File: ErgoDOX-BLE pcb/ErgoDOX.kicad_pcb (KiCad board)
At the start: 2 copper layers, 182.8 x 158.9 mm, 110 parts, among them J1 Conn_01x04, J2 Conn_01x02_Female, J3 Conn_01x02_Female, J4 Conn_01x02, J5 Conn_01x02, P1 USB_C_Plug_USB2.0, Q1 Q_NPN_BCE, SW0:10 SW0:3, SW0:11 SW0:2, SW0:12 SW0:1, SW0:7 SW0:6, SW0:8 SW0:5, SW0:9 SW0:4, SW1:10 SW1:3, SW1:11 SW1:2, SW1:12 SW1:1, SW1:13 SW1:0, SW1:9 SW1:4, SW2:10 SW2:3, SW2:11 SW2:2, SW2:12 SW2:1, SW2:13 SW2:0, SW2:7 SW2:6, SW2:8 SW2:5, SW2:9 SW2:4, SW3:10 SW3:3, SW3:11 SW3:2, SW3:12 SW3:1, SW3:13 SW3:0, SW3:8 SW3:5, SW3:9 SW3:4, SW4:10 SW4:3, SW4:11 SW4:2, SW4:12 SW4:1, SW4:13 SW4:0, SW4:7 SW4:6, SW4:8 SW4:5, SW4:9 SW4:4, SW5:10 SW5:3, SW5:11 SW5:2, SW5:12 SW5:1, SW5:13 SW5:0, SW5:7 SW5:6, SW5:8 SW5:5, SW5:9 SW5:4, U1 MCP23018, U3 C0720B001F

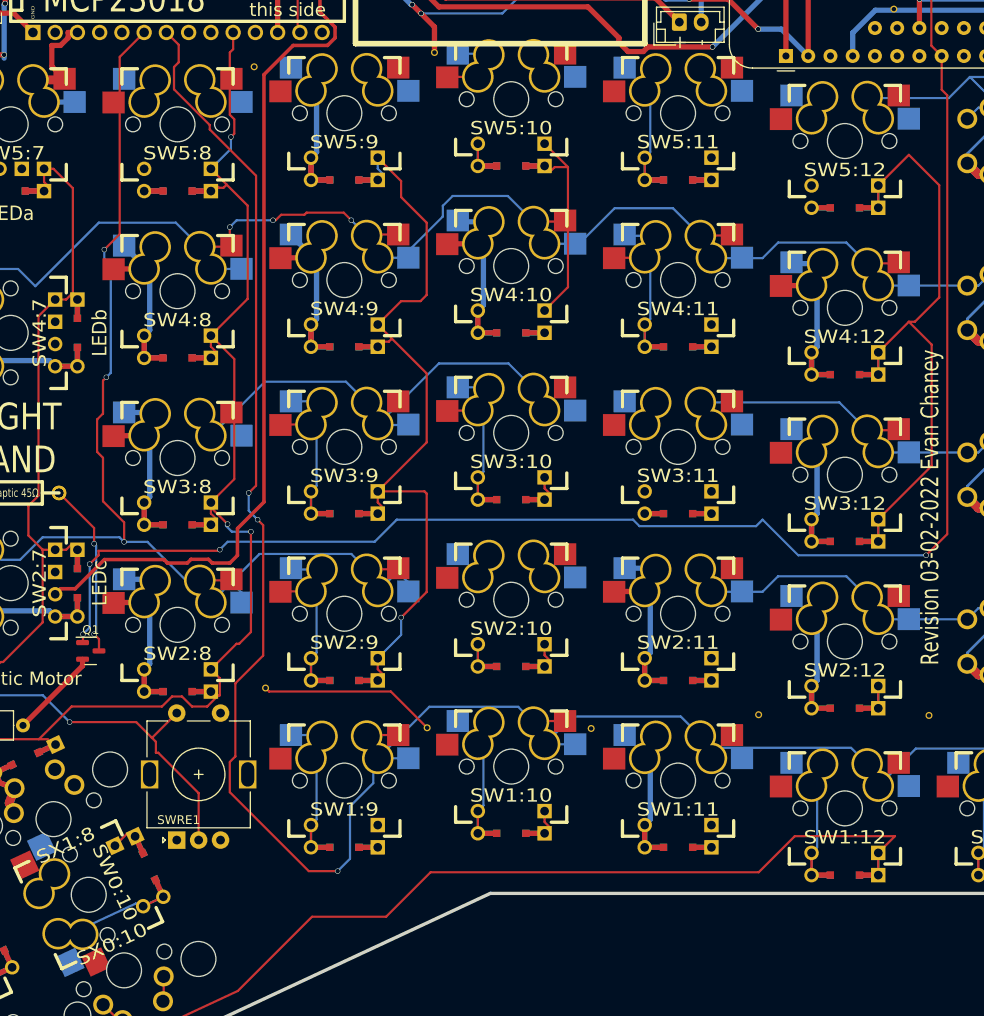
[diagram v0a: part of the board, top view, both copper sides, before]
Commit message: Restart my routing mess
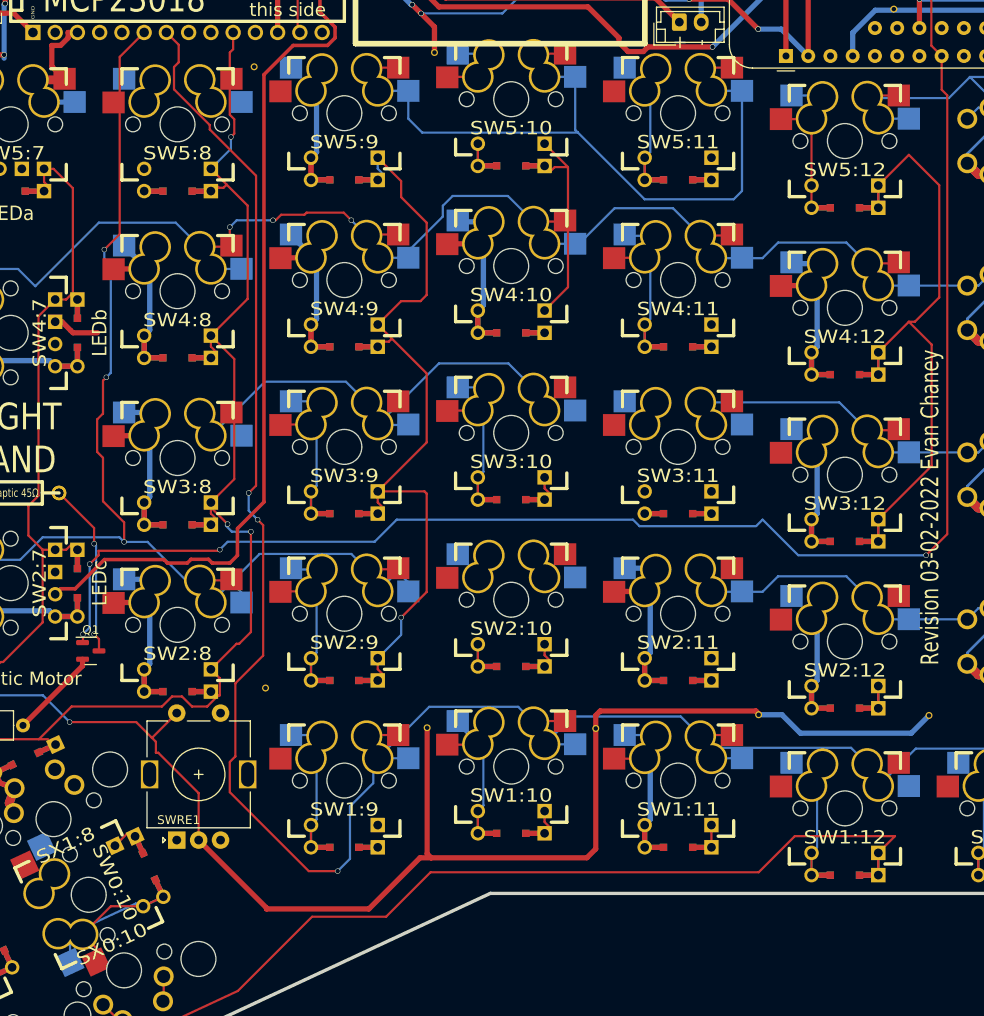
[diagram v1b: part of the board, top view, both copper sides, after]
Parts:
- moved STITCHING_VIA 0.52 mm to (139.2, 134.1)
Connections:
- STITCHING_VIA pad GND: /COL5 -> (no net)
- STITCHING_VIA pad GND: /COL5 -> GND
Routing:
- net GND: track 266.9 -> 394.3 mm
- net /ROW5: track 66.1 -> 158.1 mm
- net /COL5: track 189.5 -> 169.1 mm
- net Net-(SW5:12-Pad2): track 0.00 -> 16.5 mm
- net Net-(SW0:10-Pad2): track 15.9 -> 31.8 mm
- net /ROW1: track 229.0 -> 236.1 mm
- net Net-(SW1:11-Pad2): track 15.9 -> 23.0 mm
- net Net-(SW1:10-Pad2): track 15.9 -> 23.0 mm
- net /COL2: track 0.00 -> 1.80 mm

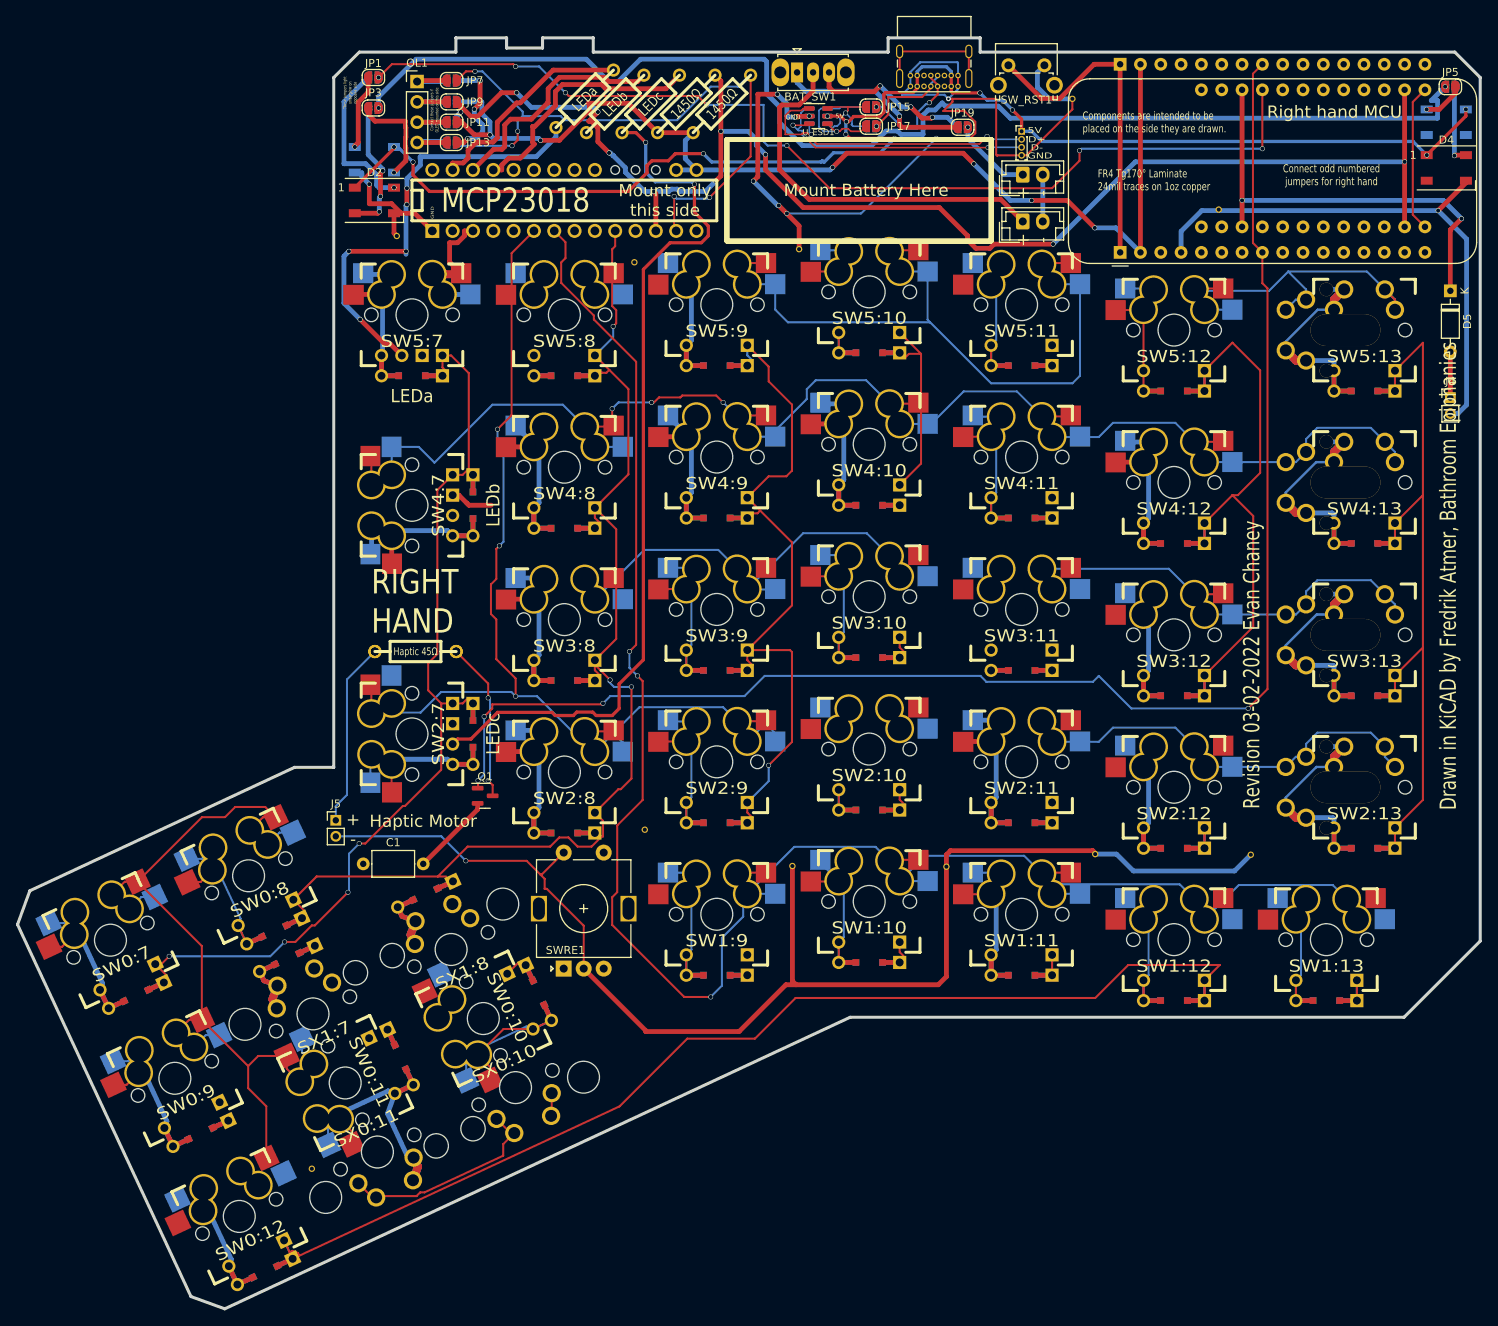
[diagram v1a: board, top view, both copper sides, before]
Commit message: More routing
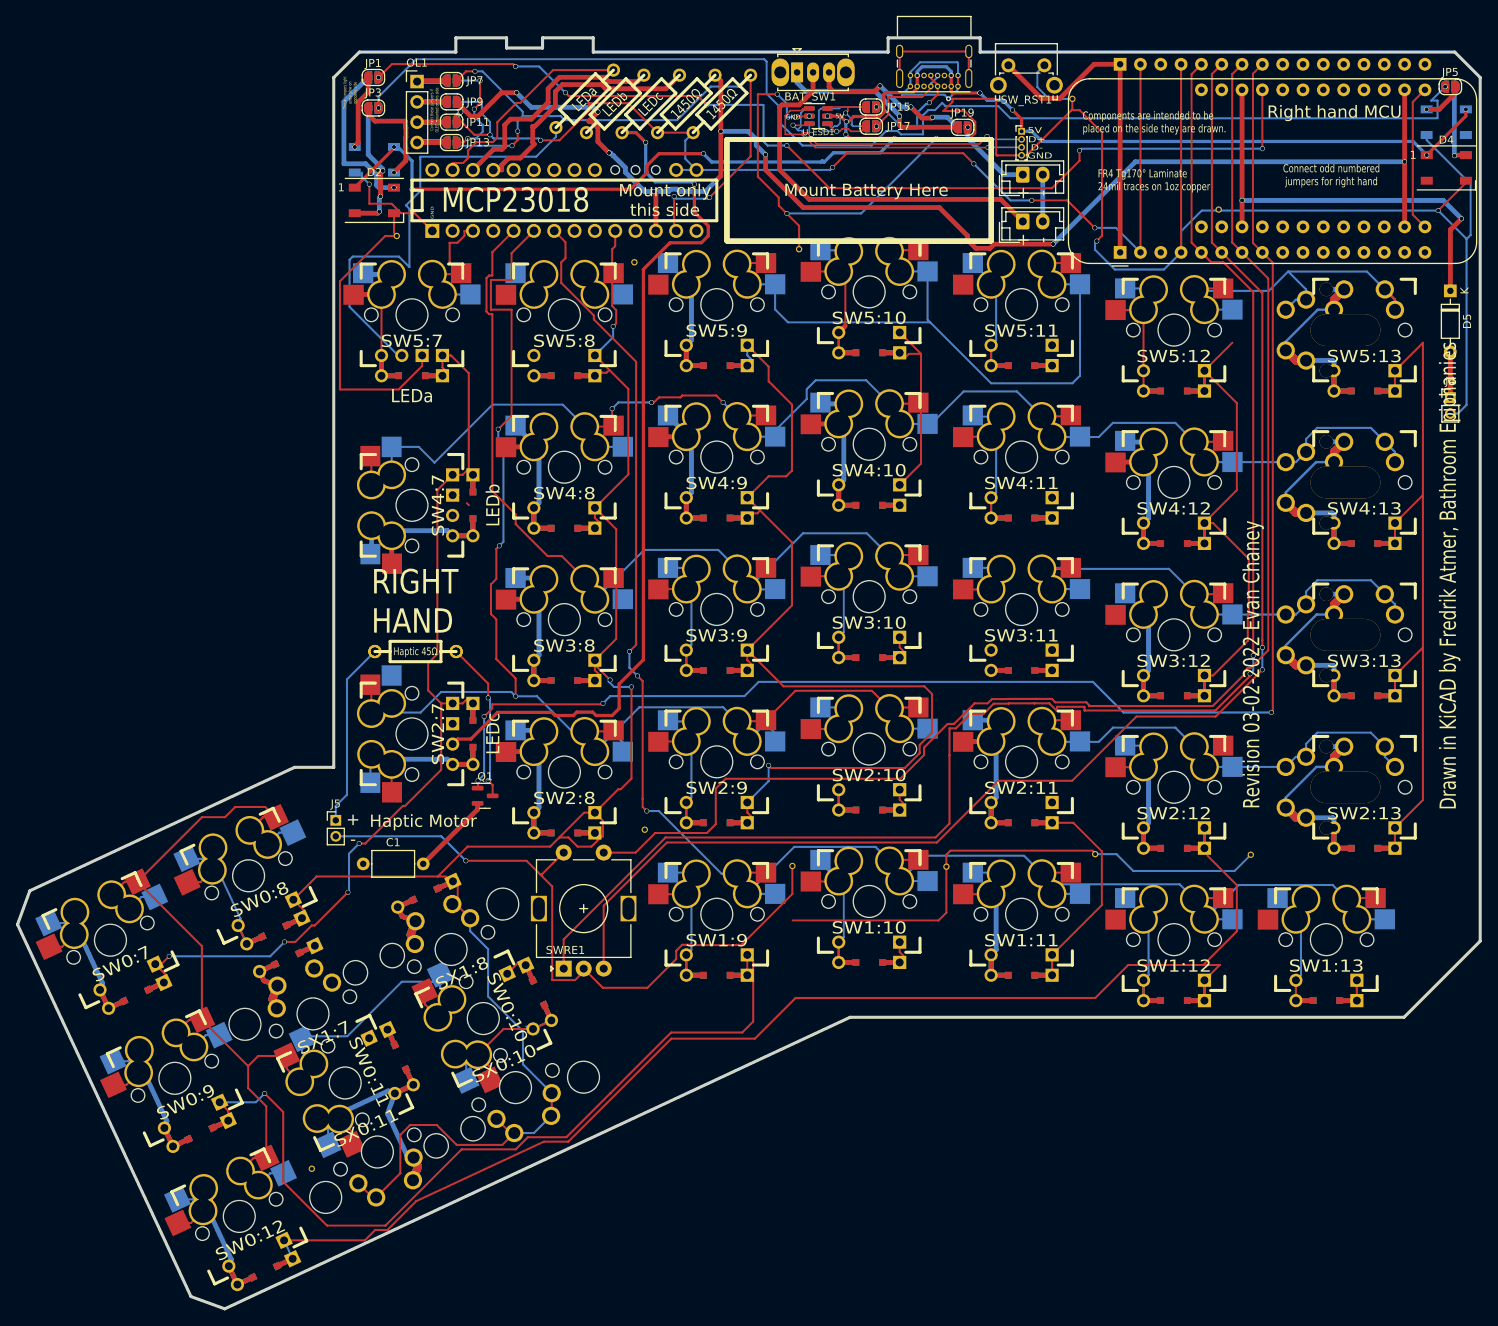
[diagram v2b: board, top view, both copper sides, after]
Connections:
- SX0:10 pad : /COL5 -> (no net)
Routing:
- net /EncoderPin1: track 0.00 -> 193.1 mm, vias 0 -> 2
- net /EncoderPin2: track 0.00 -> 181.2 mm, vias 0 -> 2
- net /EncoderClick: track 0.00 -> 173.4 mm
- net /COL4: track 83.1 -> 217.4 mm, vias 1 -> 2
- net GND: track 394.3 -> 482.5 mm, vias 14 -> 13
- net /ROW3: track 107.7 -> 173.6 mm
- net /COL5: track 169.1 -> 216.8 mm
- net /ROW0: track 103.9 -> 139.8 mm
- net /ROW2: track 184.7 -> 218.5 mm
- net /COL2: track 1.80 -> 24.3 mm
- net /ROW1: track 236.1 -> 219.3 mm
- net /COL1: track 218.7 -> 230.9 mm
- net Net-(SW5:10-Pad2): track 12.7 -> 21.0 mm
- net Net-(SW0:12-Pad2): track 15.9 -> 23.5 mm
- net Net-(SW2:12-Pad2): track 15.9 -> 23.0 mm
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
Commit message: More routing forever
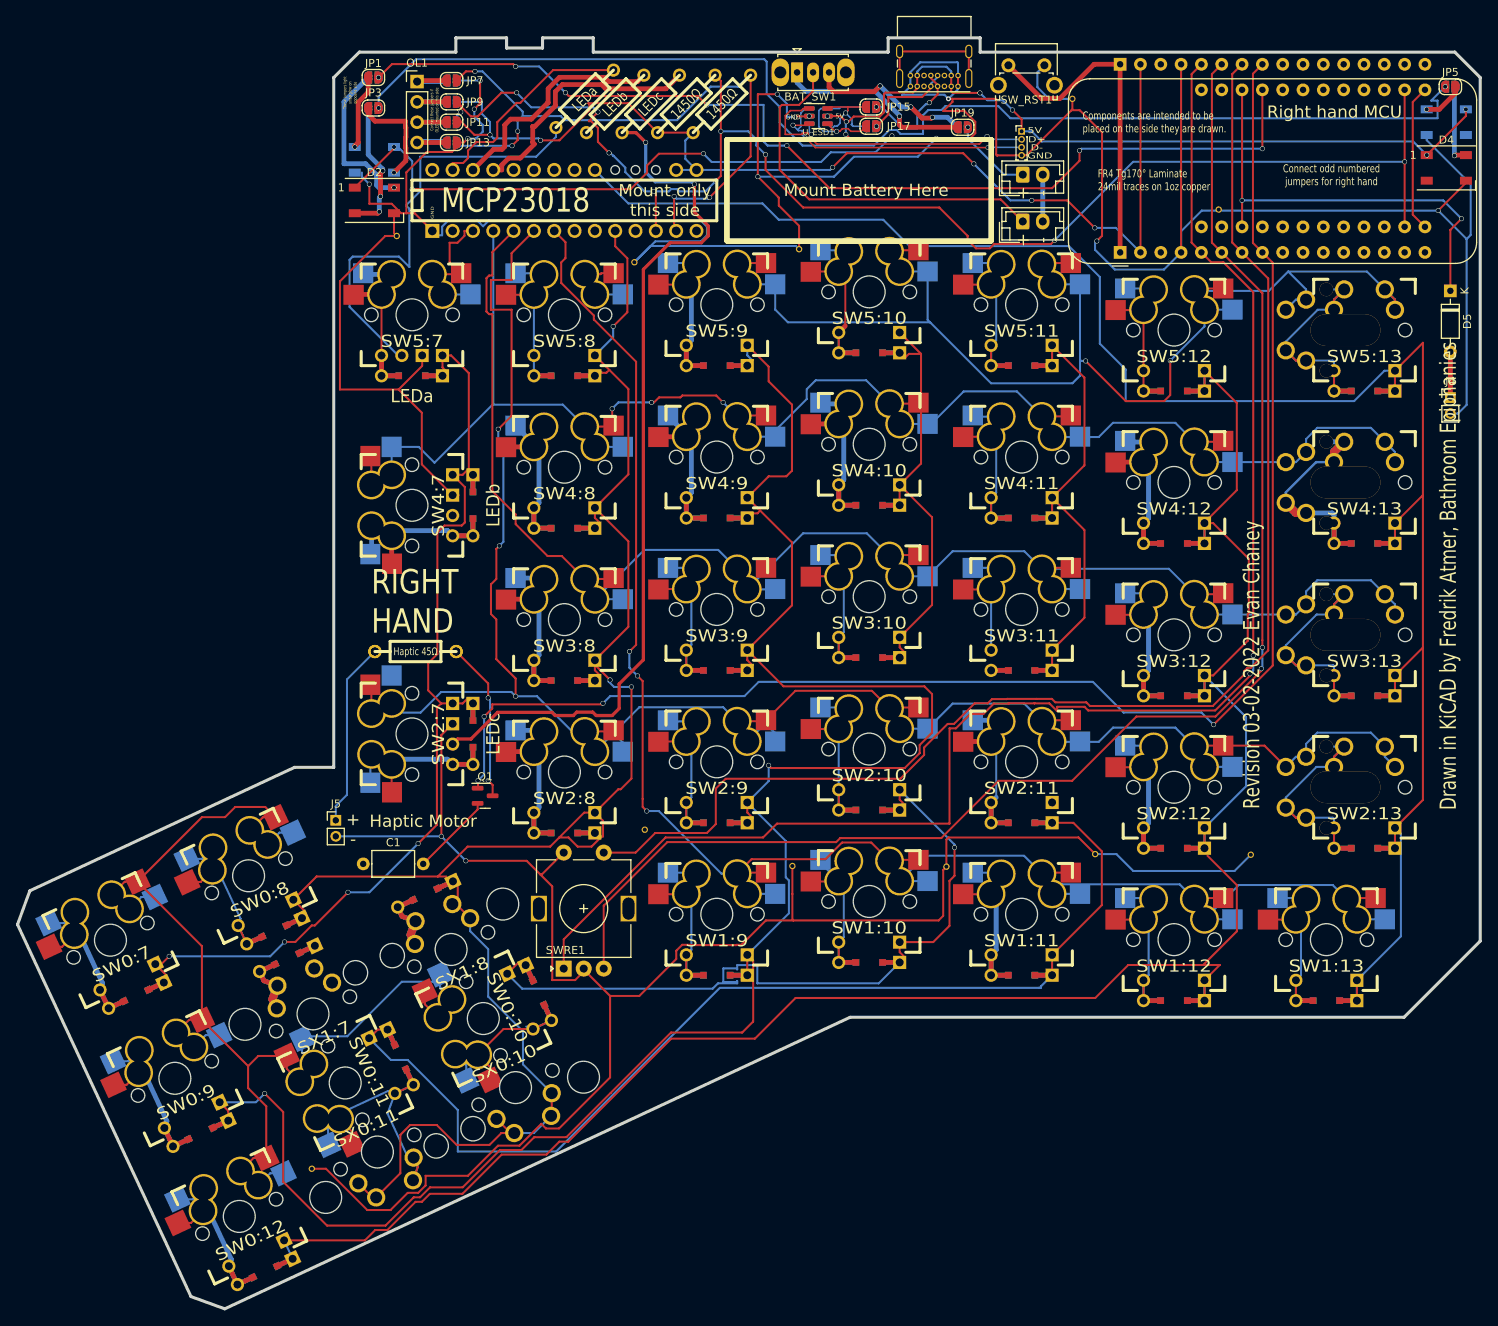
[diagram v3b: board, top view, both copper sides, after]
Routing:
- net GND: track 482.5 -> 660.8 mm, vias 13 -> 14
- net /COL2: track 24.3 -> 179.1 mm
- net /COL0: track 102.3 -> 244.7 mm
- net /COL3: track 32.0 -> 142.0 mm, vias 0 -> 1
- net /ROW5: track 158.1 -> 191.5 mm, vias 0 -> 2
- net /ROW3: track 173.6 -> 197.2 mm
- net /COL4: track 217.4 -> 240.6 mm
- net /ROW2: track 218.5 -> 240.9 mm
- net /ROW4: track 177.3 -> 199.1 mm
- net /COL1: track 230.9 -> 250.7 mm
- net Net-(SW5:8-Pad2): track 0.00 -> 16.5 mm
- net Net-(SW3:11-Pad2): track 7.12 -> 14.7 mm
- net Net-(SW2:10-Pad2): track 15.8 -> 23.4 mm
- net Net-(SW1:12-Pad2): track 15.9 -> 23.0 mm
- net Net-(SW3:12-Pad2): track 15.9 -> 23.0 mm
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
